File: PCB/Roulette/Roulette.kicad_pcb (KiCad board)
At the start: 2 copper layers, 248 parts, among them J1 USB-C, J2 Shelly, J3 USB-PROG, SW1 SW_Push, U1 ESP32-S3-MINI-1, U2 MD8942

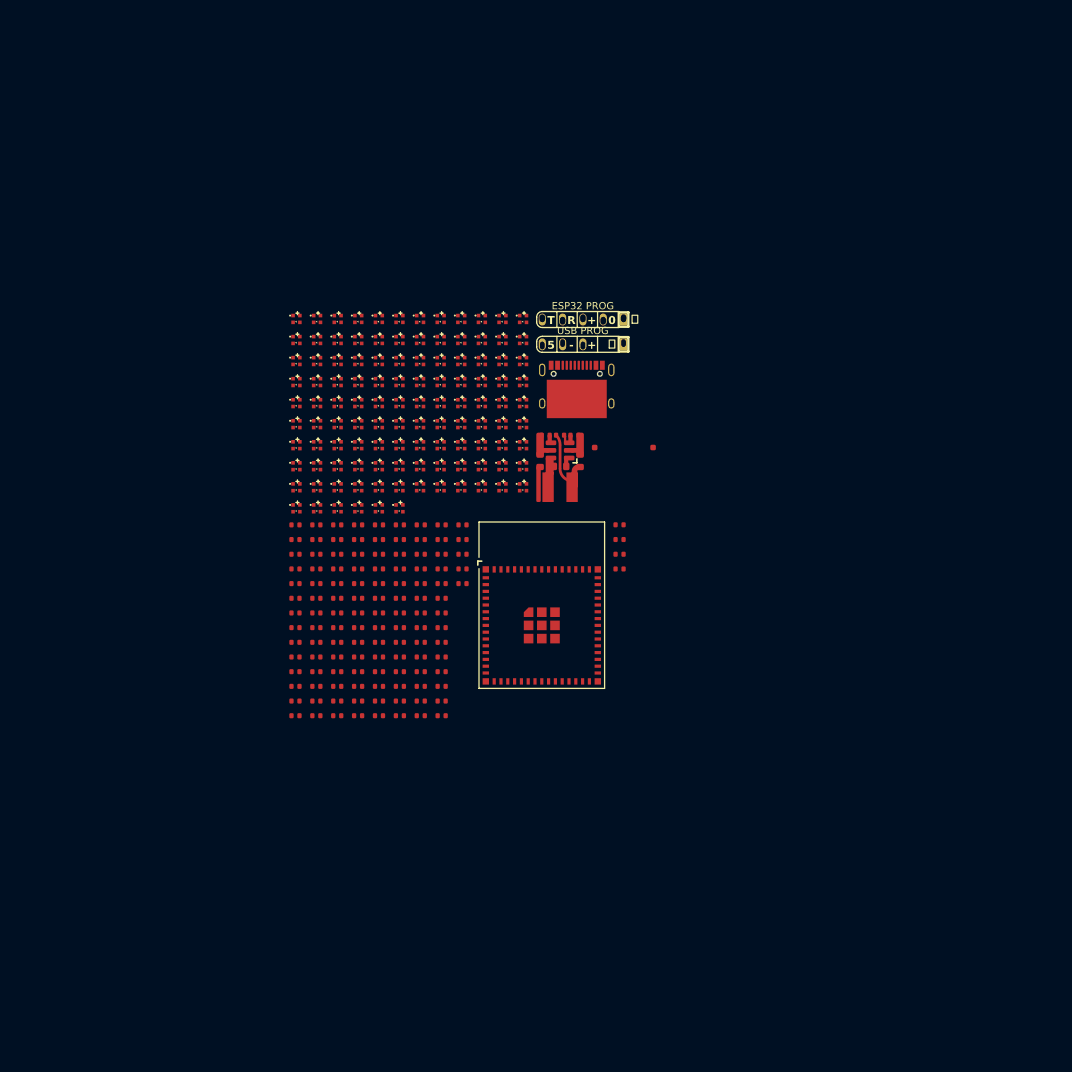
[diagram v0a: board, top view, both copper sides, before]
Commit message: Started
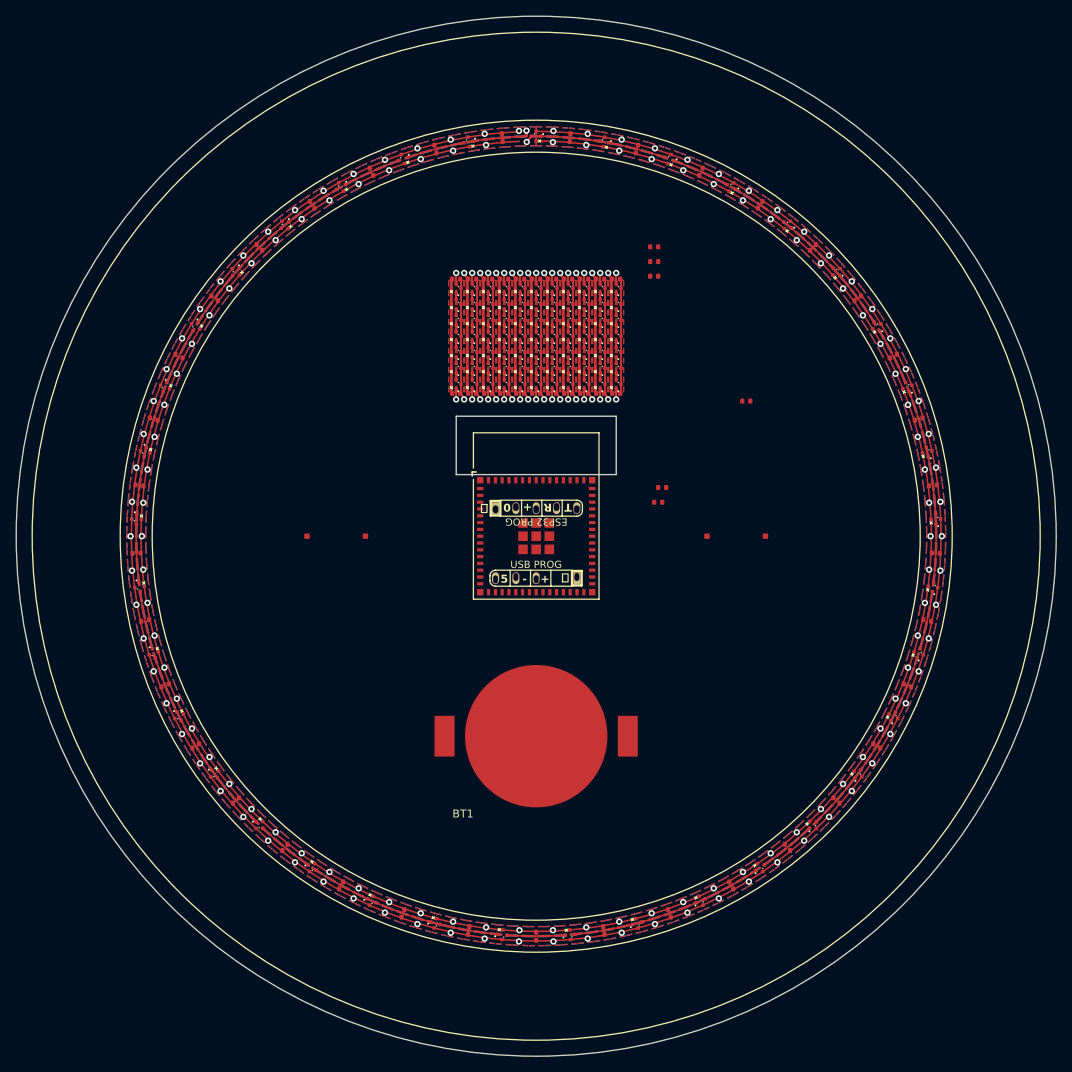
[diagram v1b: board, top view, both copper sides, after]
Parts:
- removed C100, C101, C102, C103, C104, C105, C106, C107, C108, C109, C110, C111, C112, C113, C114, C115, C116, C117, C118, C119, C120, C63, C64, C65, C66, C67, C68, C69, C70, C71, C72, C73, C74, C75, C76, C77, C78, C79, C80, C81, C82, C83, C84, C85, C86, C87, C88, C89, C90, C91, C92, C93, C94, C95, C96, C97, C98, C99: 100nF, RevK:C_0402
- removed J3: USB-PROG, RevK:USB-PROG
- removed L1: 10uH, RevK:L_4x4_
- removed R4: 10K, RevK:R_0402
- removed R5: 124k, RevK:R_0402_
- removed R6: 39k2, RevK:R_0402_
- removed R7: 1M, RevK:R_0402_
- removed U2: MD8942, RevK:SOT-23-6-MD8942
- added BT1: Battery_Cell, RevK:Battery-Holder-2032, F.Cu at (100.0, 125.0)
- added SW2: SW_Push, RevK:TS-1092S-B3D2-G, F.Cu at (75.0, 100.0)
- C2: value 22uF -> 100nF
- C3: value 1uF -> 100nF
- C4: value 10uF 50V -> 100nF; footprint RevK:C_0603_ -> RevK:C_0402
- C5: value 10uF 6.3V -> 100nF; footprint RevK:C_0603_ -> RevK:C_0402
- C6: footprint RevK:C_0603_ -> RevK:C_0402
- C61: value 100nF -> 22uF
- C62: value 100nF -> 1uF
- J1: value USB-C -> Shelly; footprint RevK:USC16-TR -> RevK:Shelly
- J2: value Shelly -> USB-PROG; footprint RevK:Shelly -> RevK:USB-PROG
- R1, R2: value 5K1 -> 10K
- moved D13 88.2 mm to (144.6, 122.5), turned to 108.243 degrees
- moved D14 86.7 mm to (140.2, 129.7), turned to 98.5135 degrees
- moved D15 84.9 mm to (134.6, 136.1), turned to 88.7838 degrees
- moved D16 82.9 mm to (128.0, 141.4), turned to 79.0541 degrees
- moved C9 80.9 mm to (149.6, 93.6), turned to 7.2973 degrees
- moved D17 80.8 mm to (120.6, 145.6), turned to 69.3243 degrees
- moved C8 80.6 mm to (147.8, 85.4), turned to 17.027 degrees
- moved C10 80.4 mm to (150.0, 102.1), turned to -2.43243 degrees
- moved C7 79.3 mm to (144.6, 77.5), turned to 26.7568 degrees
- moved C11 79.0 mm to (148.9, 110.5), turned to -12.1622 degrees
- moved D18 78.7 mm to (112.6, 148.4), turned to 59.5946 degrees
- moved D19 76.7 mm to (104.2, 149.8), turned to 49.8649 degrees
- moved C12 76.7 mm to (146.4, 118.6), turned to -21.8919 degrees
- moved D20 74.7 mm to (95.8, 149.8), turned to 40.1351 degrees
- moved C13 73.5 mm to (142.6, 126.2), turned to -31.6216 degrees
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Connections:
- C1 pad 1: +3V3 -> VCC
- C2 pad 1: +3V3 -> VCC
- C3 pad 1: Net-(U1-EN) -> VCC
- C60 pad 1: VCC -> +3V3
- C61 pad 1: VCC -> +3V3
- C62 pad 1: VCC -> Net-(U1-EN)
- J2 pad 1: GND -> DC
- J2 pad 2: Net-(J2-0) -> D-
- J2 pad 3: +3V3 -> D+
- J2 pad 4: Net-(J2-Rx) -> GND
- R1 pad 1: Net-(J1-CC1) -> +3V3
- R1 pad 2: GND -> Net-(U1-EN)
- R2 pad 1: GND -> +3V3
- R2 pad 2: Net-(J1-CC2) -> BUTTON2
- R3 pad 2: Net-(U1-EN) -> BUTTON1
- SW1 pad 1: BUTTON -> BUTTON2
- U1 pad 28: BUTTON -> BUTTON1
- U1 pad 29: unconnected-(U1-GPIO34-Pad29) -> BUTTON2
- U1 pad 39: Net-(J2-Tx) -> Net-(J1-Tx)
- U1 pad 4: Net-(J2-0) -> Net-(J1-0)
- U1 pad 40: Net-(J2-Rx) -> Net-(J1-Rx)
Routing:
- net GND: track 0.00 -> 1010.2 mm, vias 0 -> 84
- net VCC: track 0.00 -> 1002.2 mm, vias 0 -> 83
- net Net-(D37-O): track 0.00 -> 14.7 mm, vias 0 -> 2
- net Net-(D93-O): track 0.00 -> 10.4 mm, vias 0 -> 2
- net Net-(D86-O): track 0.00 -> 10.4 mm, vias 0 -> 2
- net Net-(D79-O): track 0.00 -> 10.4 mm, vias 0 -> 2
- net Net-(D72-O): track 0.00 -> 10.4 mm, vias 0 -> 2
- net Net-(D65-O): track 0.00 -> 10.4 mm, vias 0 -> 2
- net Net-(D58-O): track 0.00 -> 10.4 mm, vias 0 -> 2
- net Net-(D51-O): track 0.00 -> 10.4 mm, vias 0 -> 2
- net Net-(D44-O): track 0.00 -> 10.4 mm, vias 0 -> 2
- net Net-(D107-O): track 0.00 -> 10.4 mm, vias 0 -> 2
- net Net-(D100-O): track 0.00 -> 10.4 mm, vias 0 -> 2
- net Net-(D6-O): track 0.00 -> 7.29 mm
- net Net-(D32-O): track 0.00 -> 7.29 mm
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- added copper zone on B.Cu, net GND
- added copper zone on F.Cu, net GND
- added copper zone on B.Cu, net VCC
- added copper zone on F.Cu, net VCC
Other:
- board outline added: 130 x 130 mm
